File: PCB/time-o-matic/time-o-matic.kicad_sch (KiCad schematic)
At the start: 31 parts, among them J1 Power from Battery, J2 USB_C_Receptacle_USB2.0_14P, J3 Power TP4056, J4 GPS connector, SW1 SW_Push, SW2 SW_Push, SW3 SW_Push, SW4 SW_Push, SW5 SW_Push, SW6 SW_Push, U1 ESP32-WROOM-E, U2 MP1584EN-LF-P, U4 CH340C

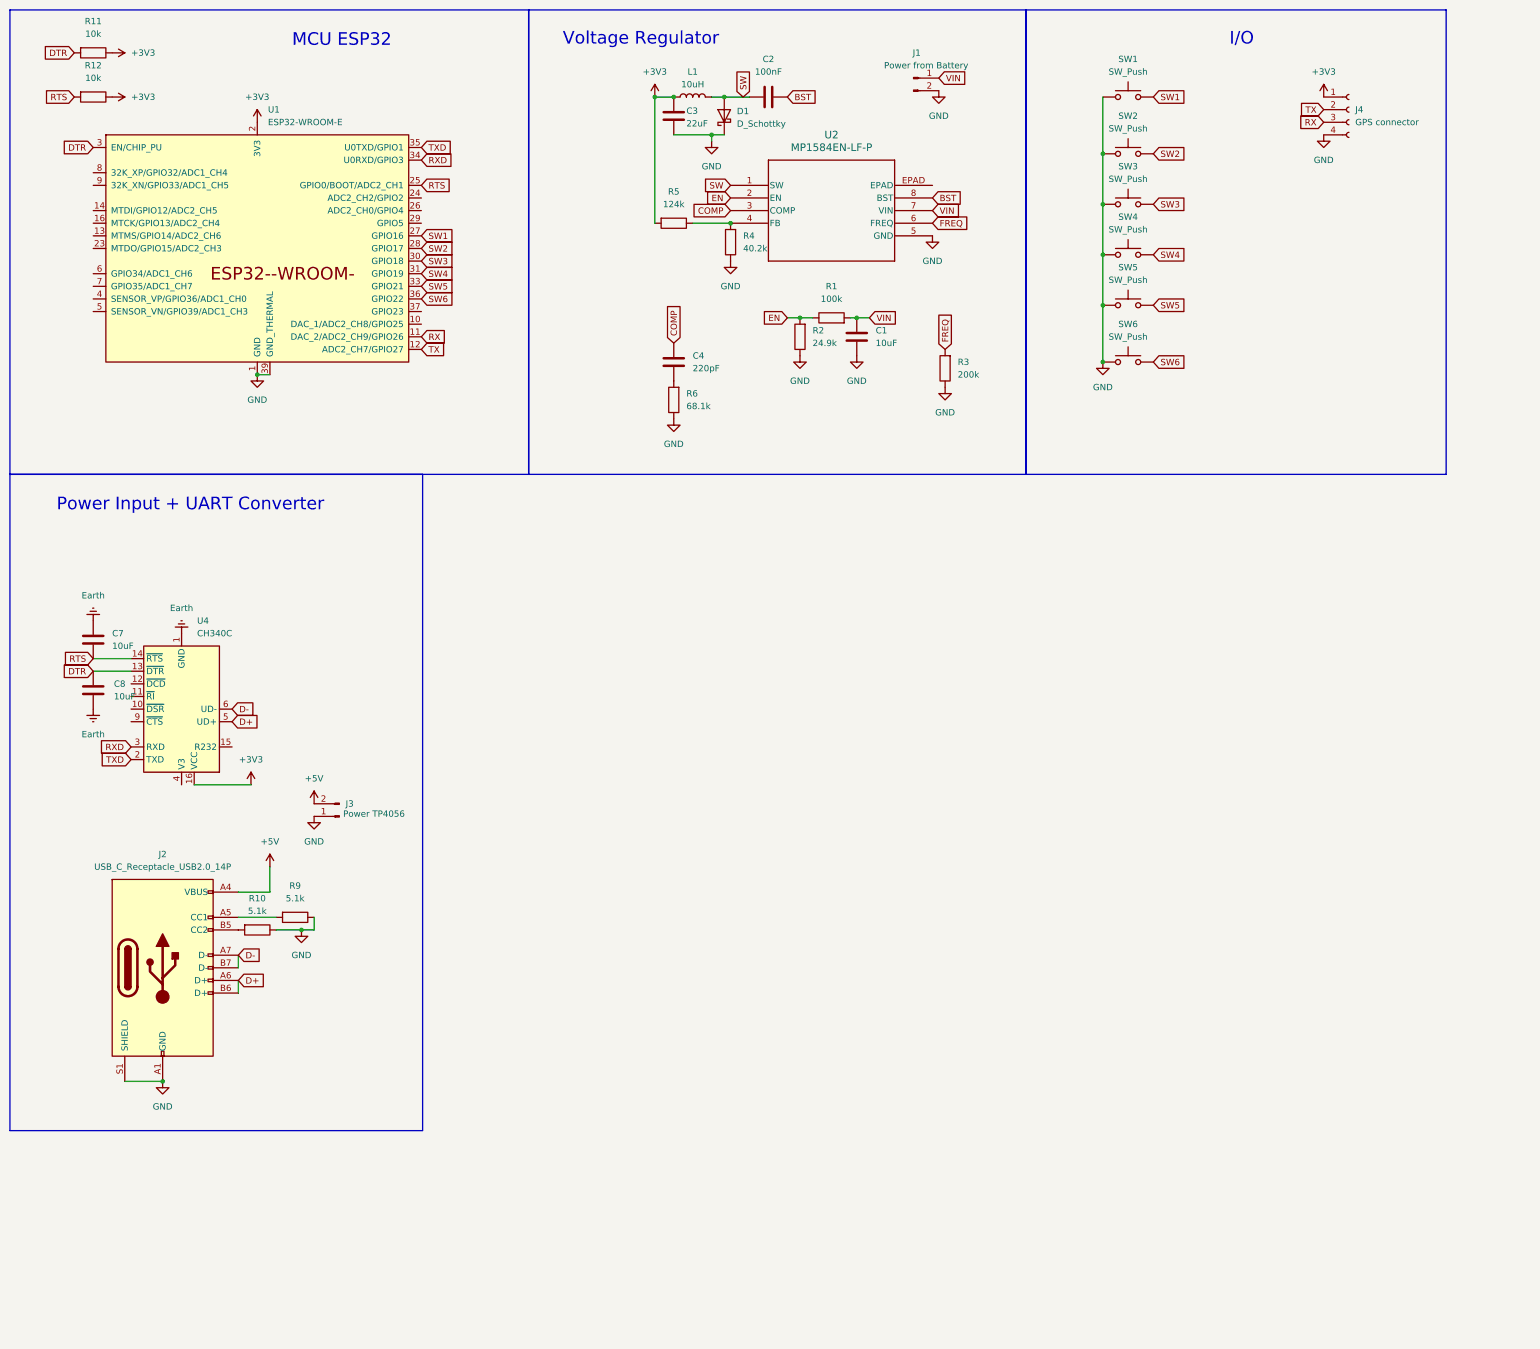
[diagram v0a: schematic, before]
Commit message: W
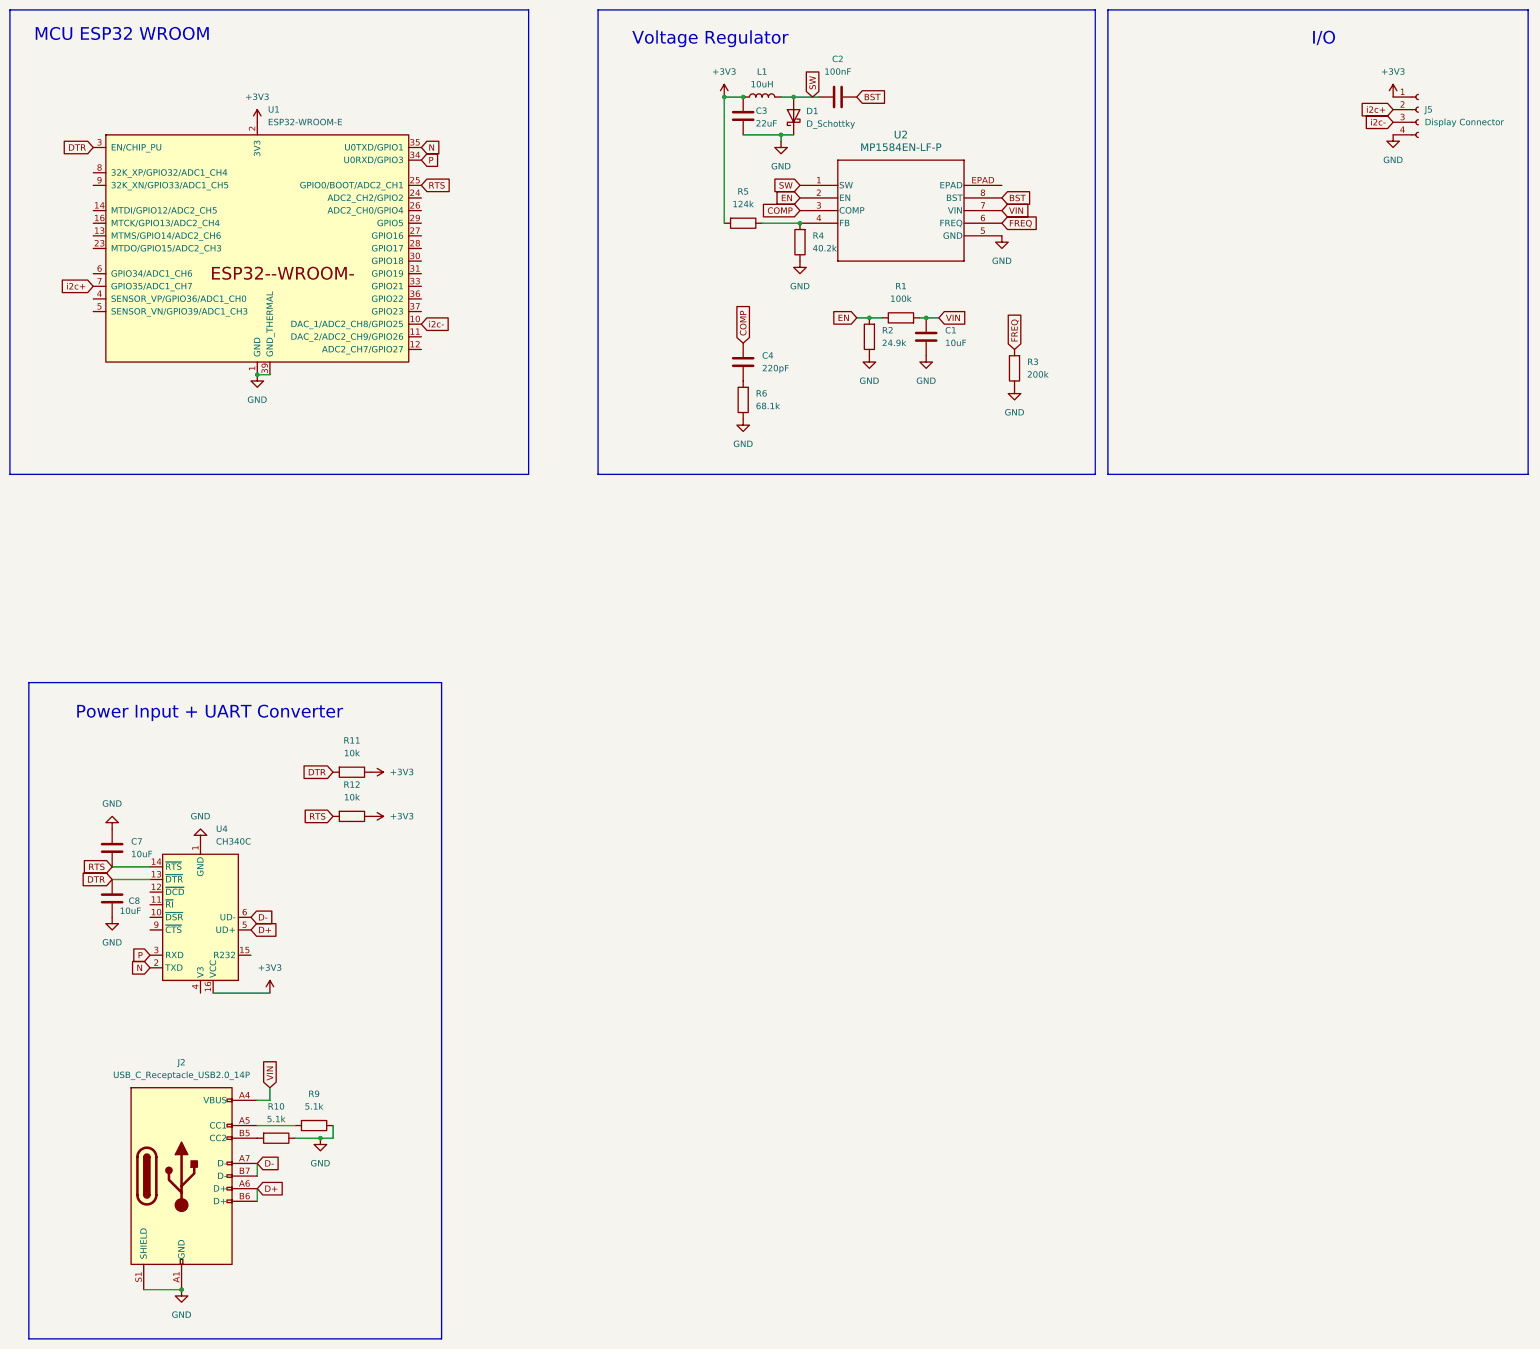
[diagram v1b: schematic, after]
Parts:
- removed J1: Power from Battery, symbol Connector:Conn_01x02_Pin
- removed J3: Power TP4056, symbol Connector:Conn_01x02_Pin
- removed J4: GPS connector, symbol Connector:Conn_01x04_Socket
- removed SW1, SW2, SW3, SW4, SW5, SW6: SW_Push, symbol Switch:SW_Push
- added J5: Display Connector, Connector_PinHeader_2.54mm:PinHeader_1x04_P2.54mm_Vertical, symbol Connector:Conn_01x04_Socket
- C1, C2, C3, C4, C7, C8: footprint (none) -> Capacitor_SMD:C_0603_1608Metric_Pad1.08x0.95mm_HandSolder
- D1: footprint (none) -> Diode_SMD:D_3220_8050Metric_Pad2.65x5.15mm_HandSolder
- J2: footprint (none) -> Connector_USB:USB_C_Receptacle_GCT_USB4085
- L1: footprint (none) -> Inductor_SMD:L_0603_1608Metric_Pad1.05x0.95mm_HandSolder
- R1, R10, R11, R12, R2, R3, R4, R5, R6, R9: footprint (none) -> Resistor_SMD:R_0603_1608Metric_Pad0.98x0.95mm_HandSolder
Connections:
- net +5V is gone; now on net VIN: J2.A4 (VBUS), J2.A9 (VBUS), J2.B4 (VBUS), J2.B9 (VBUS)
- net Earth is gone; now on net GND: C7.2, C8.1, U4.1 (GND)
- net +3V3: now also J5.1 (Pin_1)
- net GND: now also J5.4 (Pin_4)
- net i2c-: now reaches U1.10 (DAC_1/ADC2_CH8/GPIO25)
- net i2c-: now also J5.3 (Pin_3)
- net i2c+: now reaches U1.7 (GPIO35/ADC1_CH7)
- net i2c+: now also J5.2 (Pin_2)
- net RX: no longer names the net of U1.11 (DAC_2/ADC2_CH9/GPIO26)
- net RXD renamed P
- net SW1: no longer names the net of U1.27 (GPIO16)
- net SW2: no longer names the net of U1.28 (GPIO17)
- net SW3: no longer names the net of U1.30 (GPIO18)
- net SW4: no longer names the net of U1.31 (GPIO19)
- net SW5: no longer names the net of U1.33 (GPIO21)
- net SW6: no longer names the net of U1.36 (GPIO22)
- net TX: no longer names the net of U1.12 (ADC2_CH7/GPIO27)
- net TXD renamed N
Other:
- note added: "MCU ESP32 WROOM"
- note removed: "MCU ESP32"
- moved on the sheet: C1, C2, C3, C4, C7, C8, D1, J2, L1, R1, R10, R11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
